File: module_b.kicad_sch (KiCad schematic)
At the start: 4 parts, among them J4 Bus_M.2_Socket_M, J8 HDMI_C_1.4

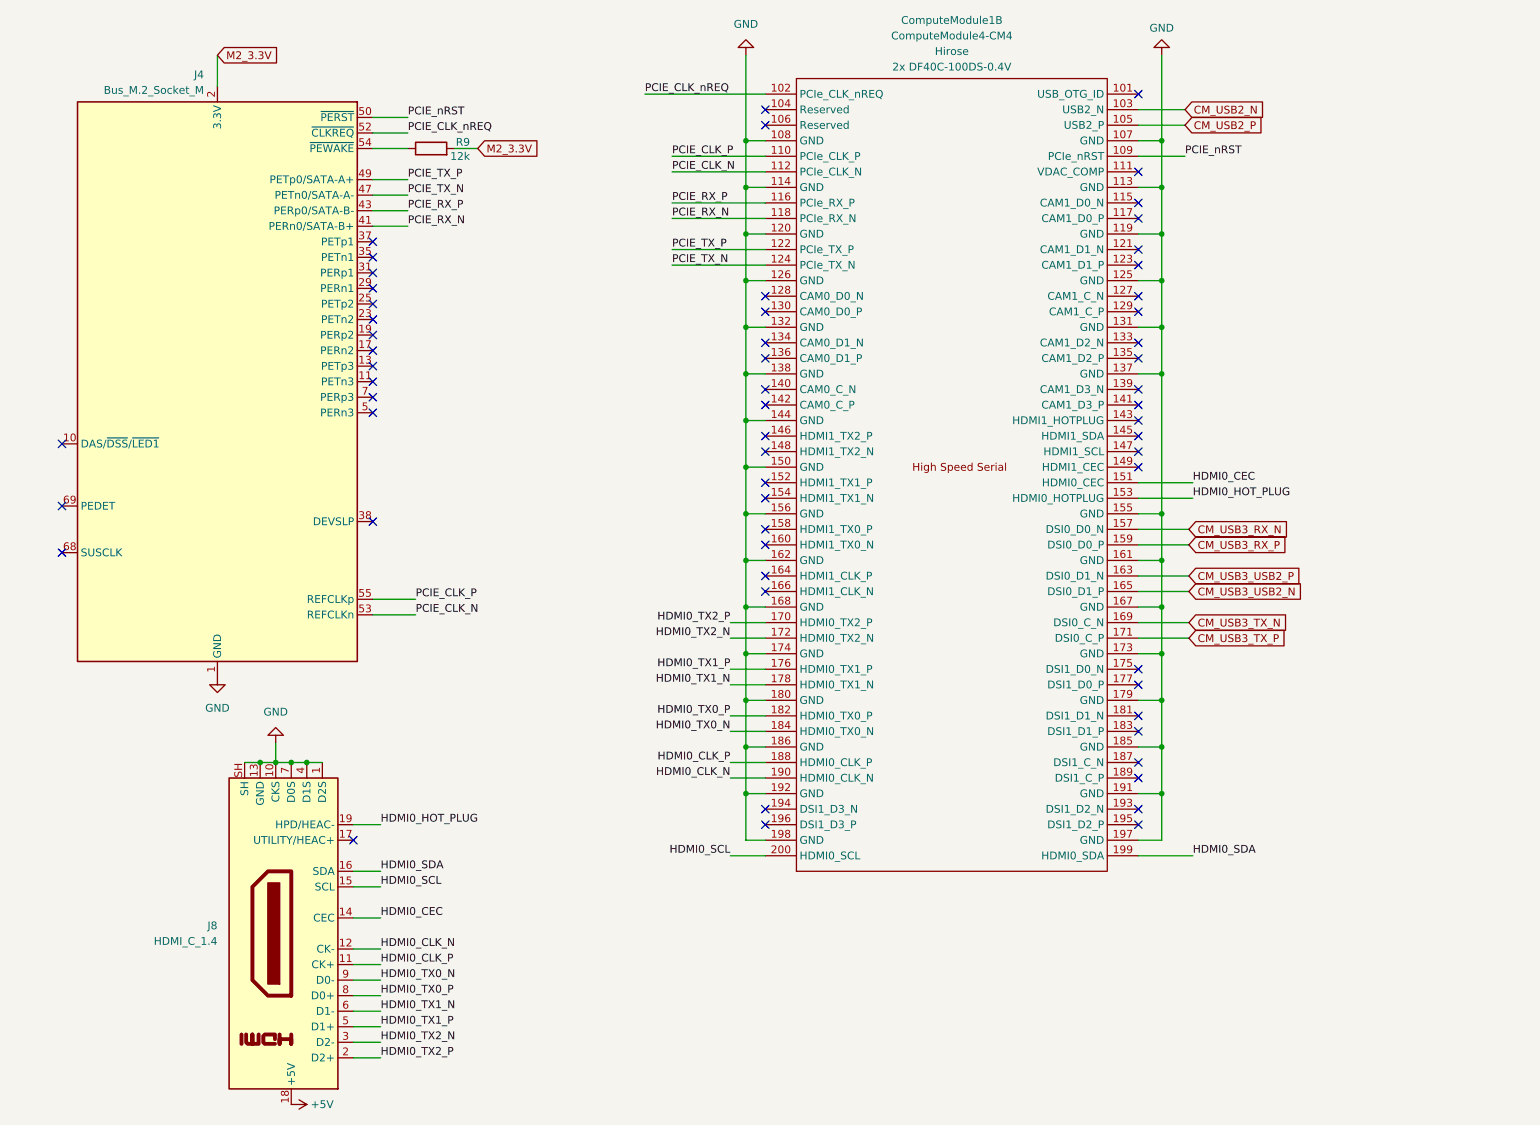
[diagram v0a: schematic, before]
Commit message: PiCard v3.0
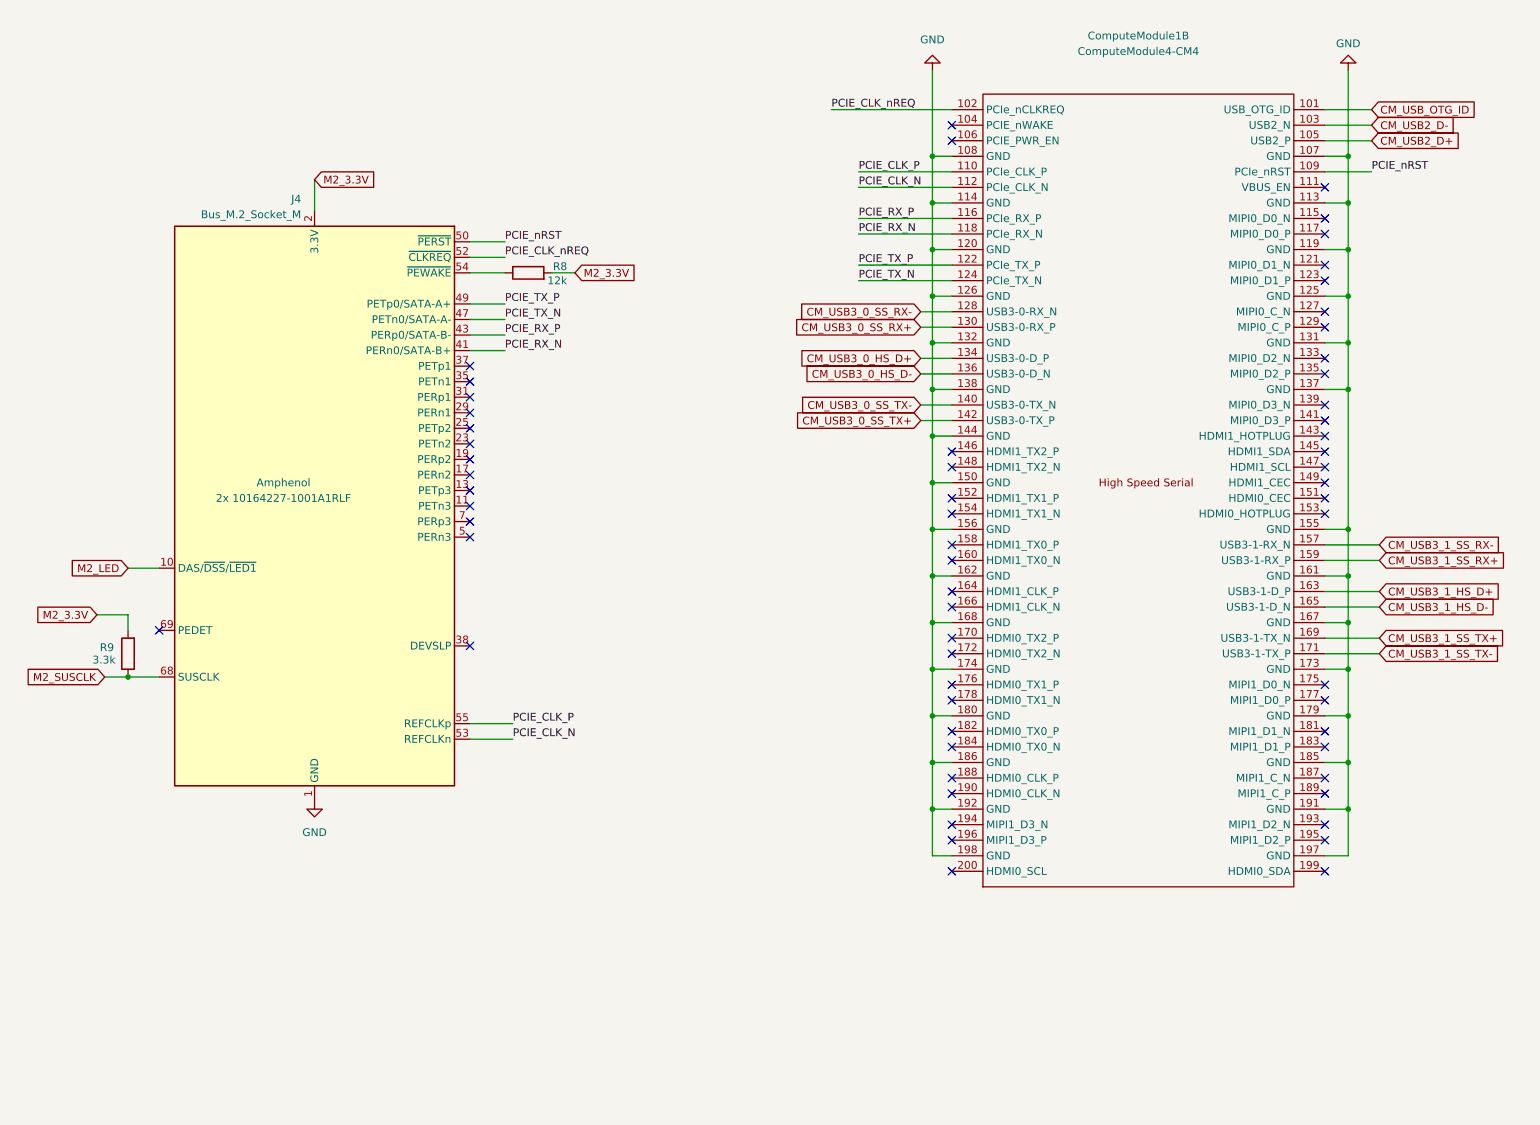
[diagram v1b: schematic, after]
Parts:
- removed J8: HDMI_C_1.4, PiCard:HDMI-SMD_19P-P0.40-H-F_HDMI-519S, symbol Connector:HDMI_C_1.4
- added R9: 3.3k, Resistor_SMD:R_0402_1005Metric, symbol Device:R
- ComputeModule1: symbol PiCard:ComputeModule4-CM4 -> PiCard:ComputeModule5-CM5; Field4 Hirose -> Amphenol; Field5 2x DF40C-100DS-0.4V -> 2x 10164227-1001A1RLF
- renumbered R9 to R8
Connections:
- net M2_3.3V: now also R9.2
- net M2_LED: now reaches J4.10 (DAS/~{DSS}/~{LED1})
- net M2_SUSCLK: now reaches J4.68 (SUSCLK)
- net M2_SUSCLK: now also R9.1
- net CM_USB_OTG_ID: now reaches ComputeModule1.101 (USB_OTG_ID)
- net CM_USB3_0_SS_RX-: now reaches ComputeModule1.128 (USB3-0-RX_N)
- net CM_USB3_0_SS_RX+: now reaches ComputeModule1.130 (USB3-0-RX_P)
- net CM_USB3_0_HS_D+: now reaches ComputeModule1.134 (USB3-0-D_P)
- net CM_USB3_0_HS_D-: now reaches ComputeModule1.136 (USB3-0-D_N)
- net CM_USB3_0_SS_TX-: now reaches ComputeModule1.140 (USB3-0-TX_N)
- net CM_USB3_0_SS_TX+: now reaches ComputeModule1.142 (USB3-0-TX_P)
- net CM_USB2_N renamed CM_USB2_D-
- net CM_USB2_P renamed CM_USB2_D+
- net CM_USB3_RX_N renamed CM_USB3_1_SS_RX-
- net CM_USB3_RX_P renamed CM_USB3_1_SS_RX+
- net CM_USB3_TX_N renamed CM_USB3_1_SS_TX+
- net CM_USB3_TX_P renamed CM_USB3_1_SS_TX-
- net CM_USB3_USB2_N renamed CM_USB3_1_HS_D-
- net CM_USB3_USB2_P renamed CM_USB3_1_HS_D+
- net HDMI0_CEC: no longer names the net of ComputeModule1.151 (HDMI0_CEC)
- net HDMI0_CLK_N: no longer names the net of ComputeModule1.190 (HDMI0_CLK_N)
- net HDMI0_CLK_P: no longer names the net of ComputeModule1.188 (HDMI0_CLK_P)
- net HDMI0_HOT_PLUG: no longer names the net of ComputeModule1.153 (HDMI0_HOTPLUG)
- net HDMI0_SCL: no longer names the net of ComputeModule1.200 (HDMI0_SCL)
- net HDMI0_SDA: no longer names the net of ComputeModule1.199 (HDMI0_SDA)
- net HDMI0_TX0_N: no longer names the net of ComputeModule1.184 (HDMI0_TX0_N)
- net HDMI0_TX0_P: no longer names the net of ComputeModule1.182 (HDMI0_TX0_P)
- net HDMI0_TX1_N: no longer names the net of ComputeModule1.178 (HDMI0_TX1_N)
- net HDMI0_TX1_P: no longer names the net of ComputeModule1.176 (HDMI0_TX1_P)
- net HDMI0_TX2_N: no longer names the net of ComputeModule1.172 (HDMI0_TX2_N)
- net HDMI0_TX2_P: no longer names the net of ComputeModule1.170 (HDMI0_TX2_P)
- no-connect marks 59 -> 61
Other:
- title: (none) -> PiCard
- moved on the sheet: ComputeModule1B, J4, R8
